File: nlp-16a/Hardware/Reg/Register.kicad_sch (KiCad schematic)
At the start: 35 parts, among them J9 Conn_01x02_Male, U10 CD74HC00, U11 CD74HC00, U12 CD74HC00, U13 CD74HC00, U14 CD74HC00, U15 CD74HC00, U16 CD74HC00, U33 CD74HC00, U34 CD74HC00, U36 CD74HC00, U9 CD74HC00

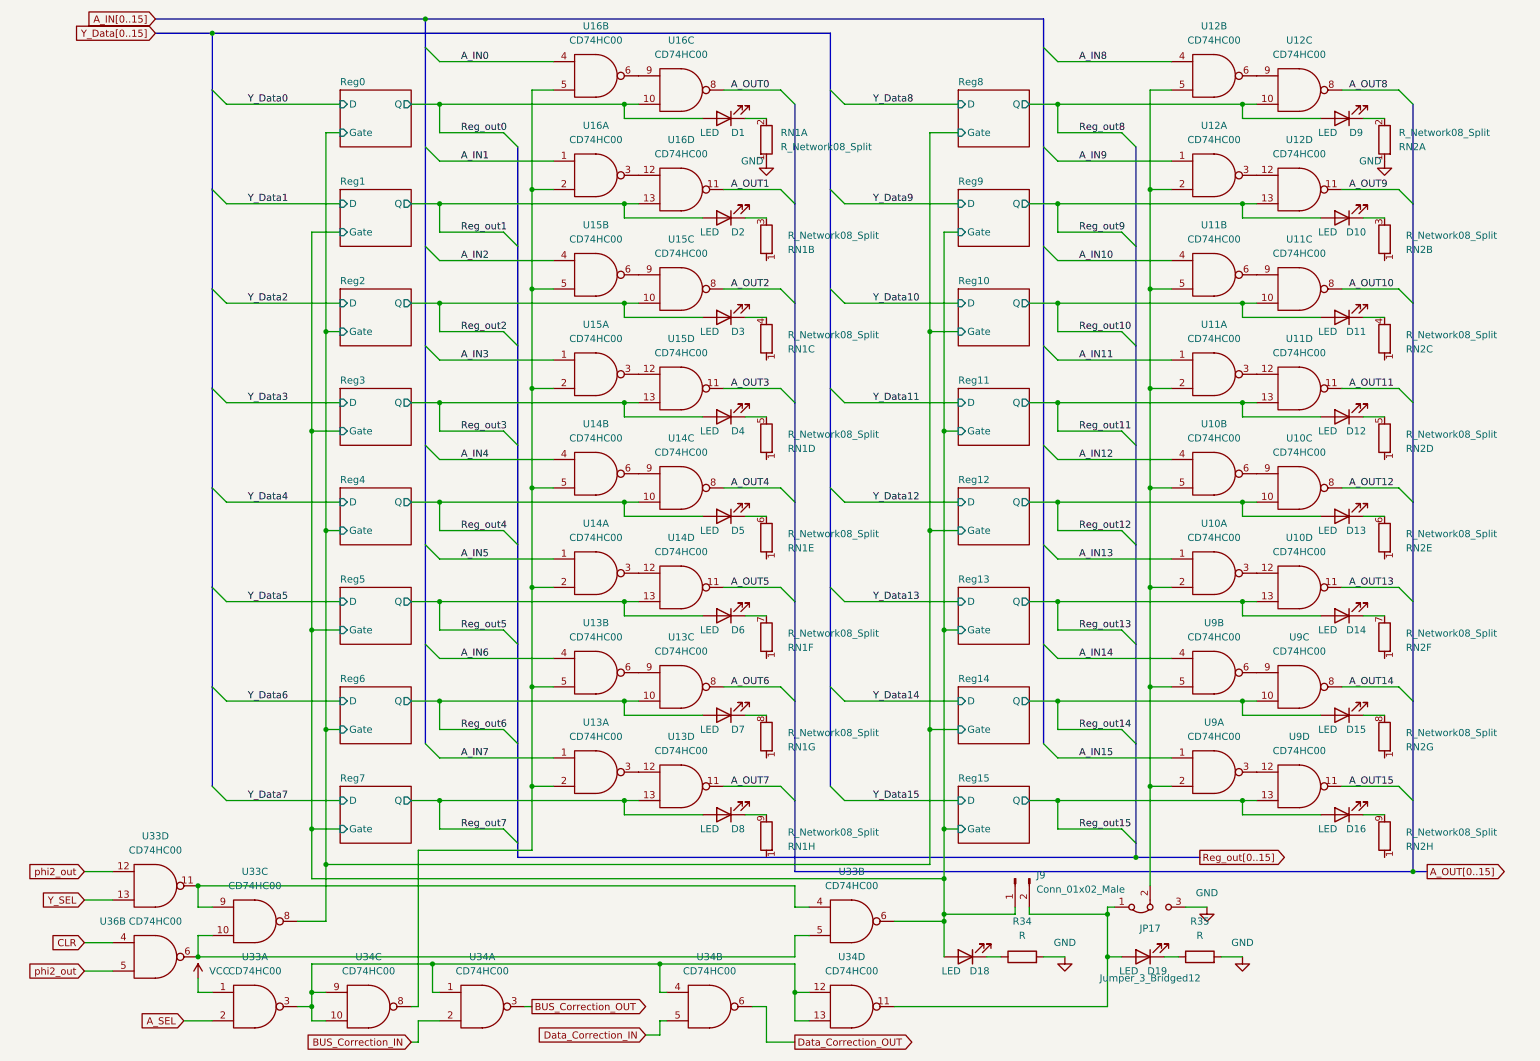
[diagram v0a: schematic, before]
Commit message: Reg更新
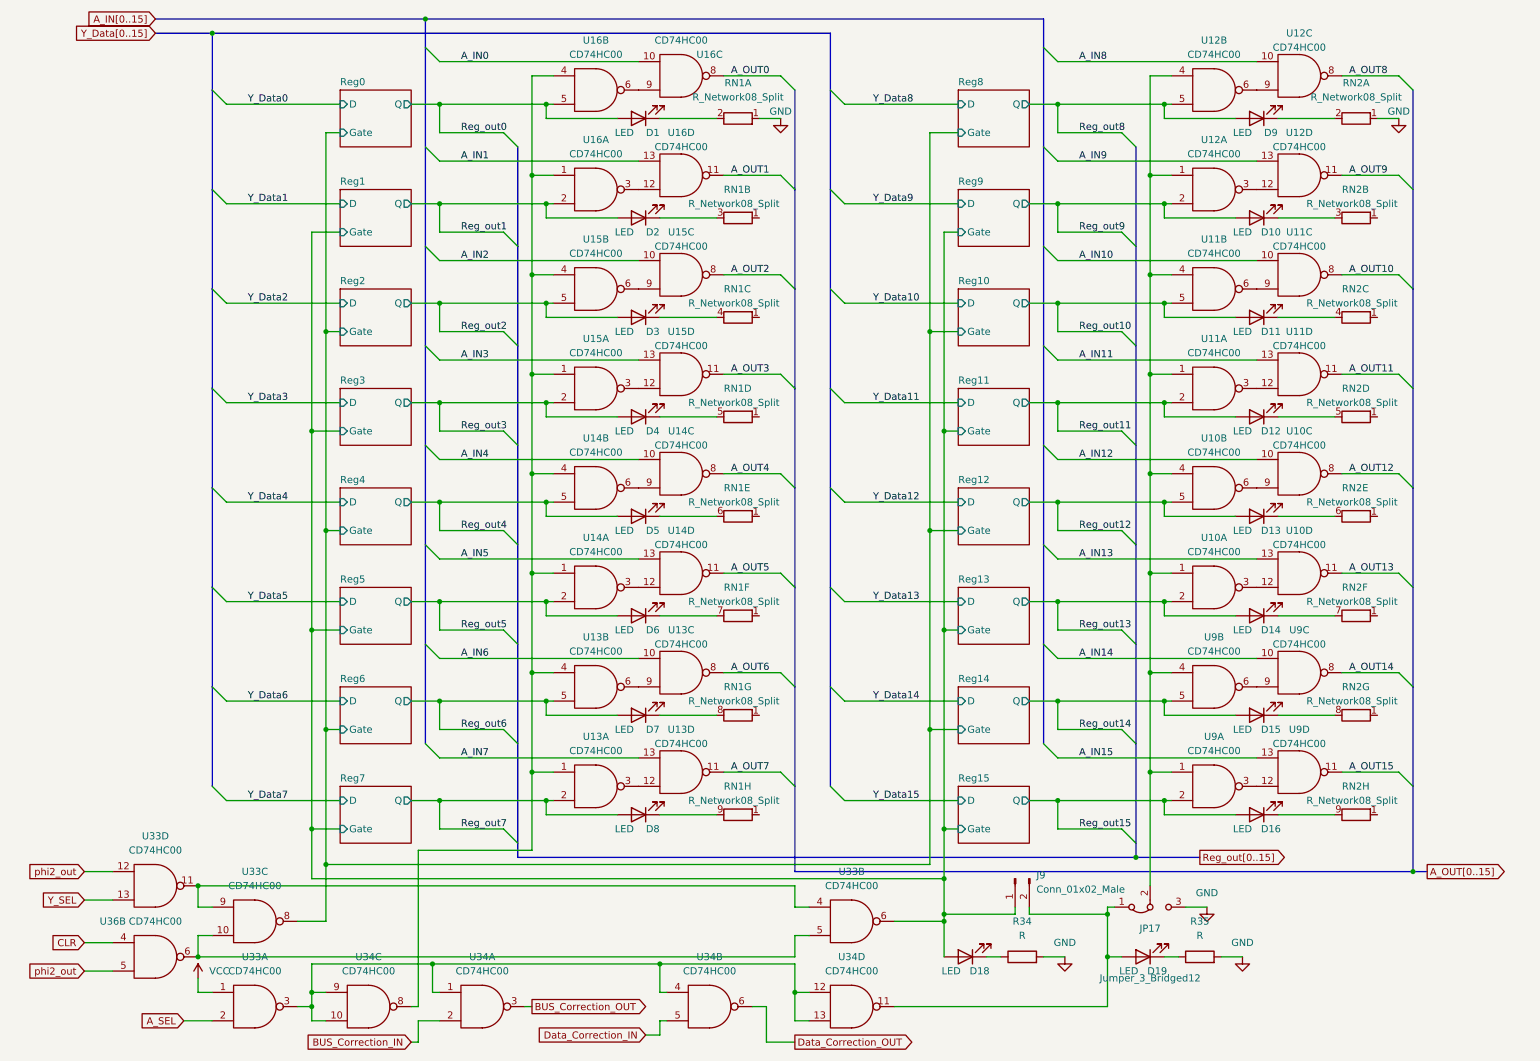
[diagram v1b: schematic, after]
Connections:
- net A_IN0: now also U16.10; no longer U16.4
- net A_IN1: now also U16.13; no longer U16.1
- net A_IN10: now also U11.10; no longer U11.4
- net A_IN11: now also U11.13; no longer U11.1
- net A_IN12: now also U10.10; no longer U10.4
- net A_IN13: now also U10.13; no longer U10.1
- net A_IN14: now also U9.10; no longer U9.4
- net A_IN15: now also U9.13; no longer U9.1
- net A_IN2: now also U15.10; no longer U15.4
- net A_IN3: now also U15.13; no longer U15.1
- net A_IN4: now also U14.10; no longer U14.4
- net A_IN5: now also U14.13; no longer U14.1
- net A_IN6: now also U13.10; no longer U13.4
- net A_IN7: now also U13.13; no longer U13.1
- net A_IN8: now also U12.10; no longer U12.4
- net A_IN9: now also U12.13; no longer U12.1
- net Reg_out0: now also U16.5; no longer U16.10
- net Reg_out1: now also U16.2; no longer U16.13
- net Reg_out10: now also U11.5; no longer U11.10
- net Reg_out11: now also U11.2; no longer U11.13
- net Reg_out12: now also U10.5; no longer U10.10
- net Reg_out13: now also U10.2; no longer U10.13
- net Reg_out14: now also U9.5; no longer U9.10
- net Reg_out15: now also U9.2; no longer U9.13
- net Reg_out2: now also U15.5; no longer U15.10
- net Reg_out3: now also U15.2; no longer U15.13
- net Reg_out4: now also U14.5; no longer U14.10
- net Reg_out5: now also U14.2; no longer U14.13
- net Reg_out6: now also U13.5; no longer U13.10
- net Reg_out7: now also U13.2; no longer U13.13
- net Reg_out8: now also U12.5; no longer U12.10
- net Reg_out9: now also U12.2; no longer U12.13
- new net: JP17.2 (C), U10.1, U10.4, U11.1, U11.4, U12.1, U12.4, U9.1, U9.4
- new net: U13.1, U13.4, U14.1, U14.4, U15.1, U15.4, U16.1, U16.4, U34.8
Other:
- moved on the sheet: D1, D10, D11, D12, D13, D14, D15, D16, D2, D3, D4, D5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
